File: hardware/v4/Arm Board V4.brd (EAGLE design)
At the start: 108 x 50.8 mm, 29 parts, among them P1 STELLARIS-LAUNCHPADSTELLARIS-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, U1 SN74LS241DW, U2 XBEE-1B3

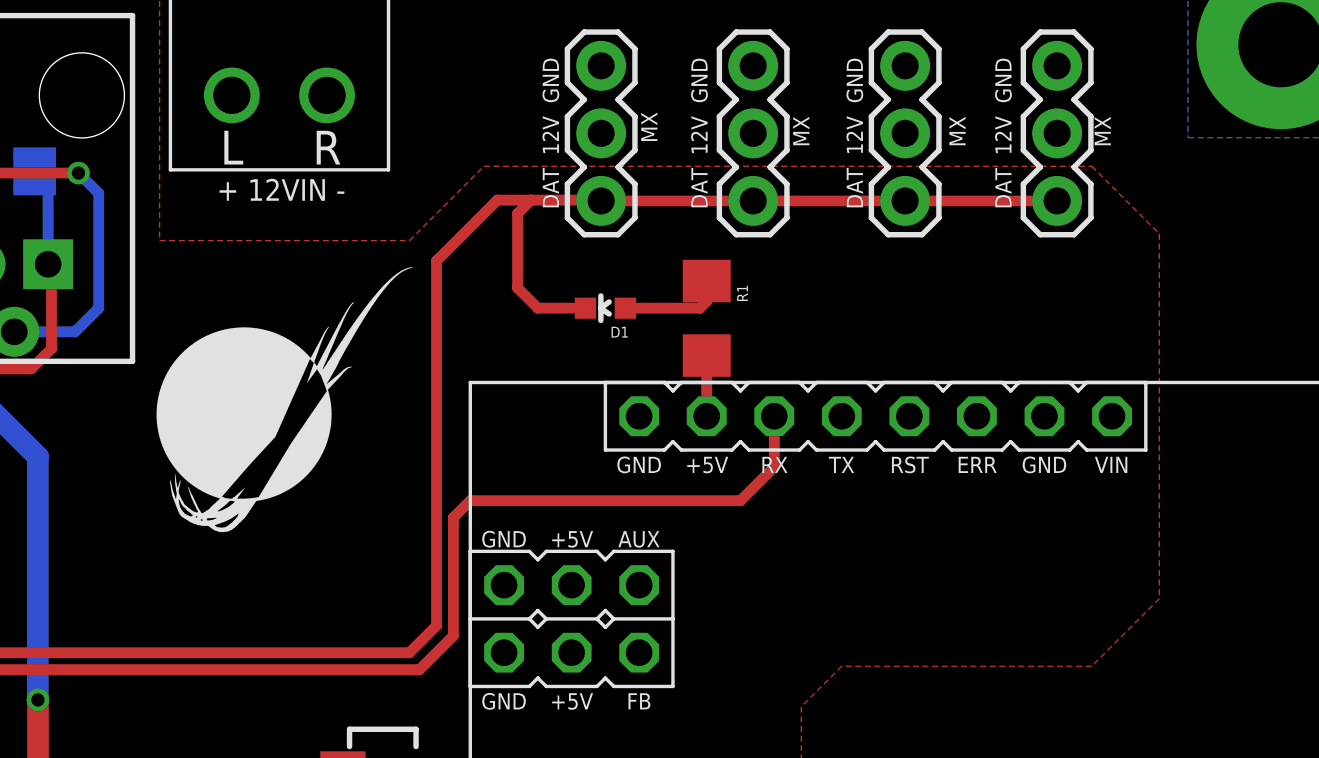
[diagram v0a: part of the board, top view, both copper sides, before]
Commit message: added refs
added BOM, jrk motor controller ds
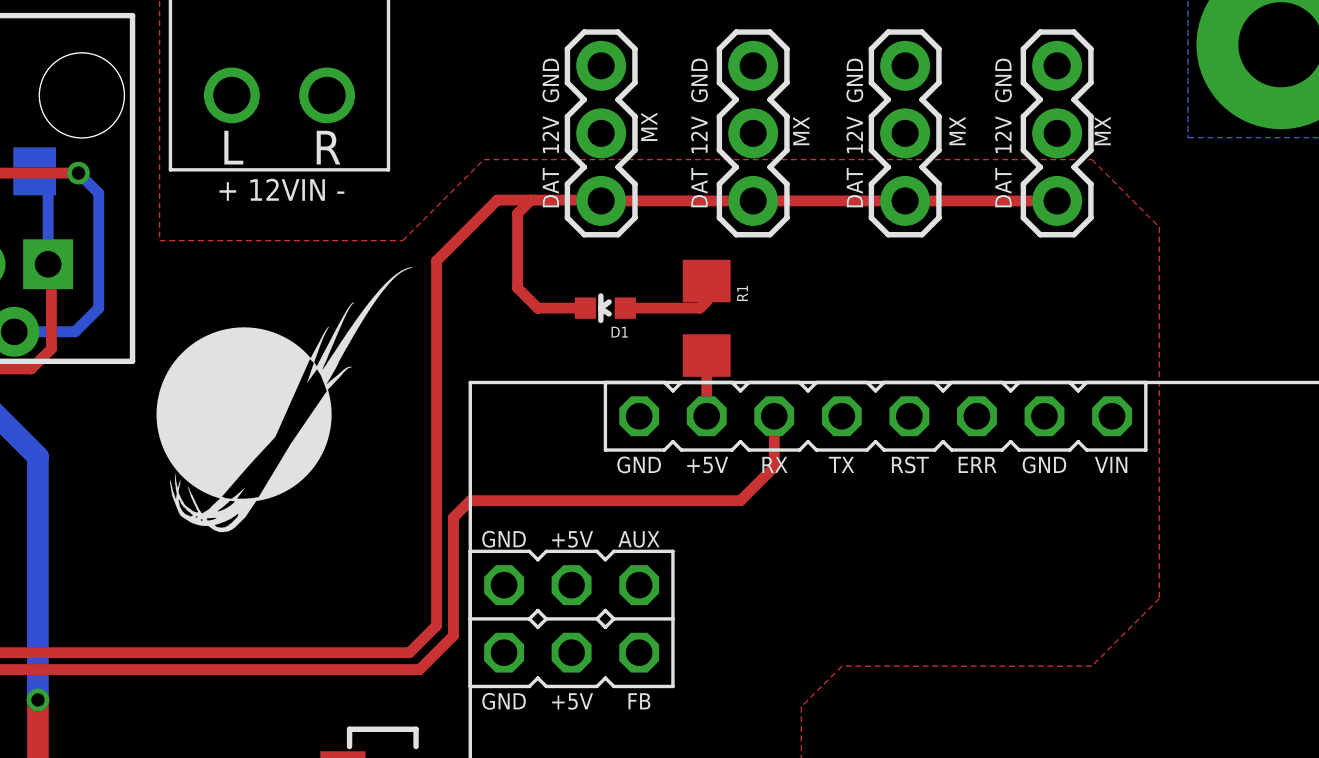
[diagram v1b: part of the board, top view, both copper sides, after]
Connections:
- net +12V: no longer U$1.VIN
- net GND: no longer U$1.GND@1
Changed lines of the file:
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@@
 <contactref element="JP2" pad="4"/>
 <contactref element="U$1" pad="GND@4"/>
-<contactref element="U$1" pad="GND@1"/>
 <polygon width="0.4064" layer="16" thermals="no">
 <vertex x="0" y="0"/>
@@
 <signal name="+12V">
 <contactref element="U$7" pad="L"/>
-<contactref element="U$1" pad="VIN"/>
 <contactref element="JP9" pad="2"/>
 <contactref element="JP10" pad="2"/>
@@
 <vertex x="61.976" y="50.8"/>
 <vertex x="61.976" y="39.624"/>
-<vertex x="71.374" y="39.624"/>
-<vertex x="74.168" y="42.418"/>
-<vertex x="97.028" y="42.418"/>
-<vertex x="99.568" y="39.878"/>
+<vertex x="71.12" y="39.624"/>
+<vertex x="74.168" y="42.672"/>
+<vertex x="97.028" y="42.672"/>
+<vertex x="99.568" y="40.132"/>
 <vertex x="99.568" y="26.162"/>
 <vertex x="97.028" y="23.622"/>
